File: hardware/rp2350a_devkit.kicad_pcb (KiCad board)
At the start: 2 copper layers, 29 x 60.5 mm, 55 parts, among them J1 USB_C_Receptacle_USB2.0_16P, J2 Conn_01x03, J3 Conn_01x16, J4 Conn_01x16, SW1 SW_Push, SW2 SW_Push, U1 NCP1117-3.3_SOT223, U2 USBLC6-2SC6, U3 W25Q128JVS, Y1 Crystal_GND24

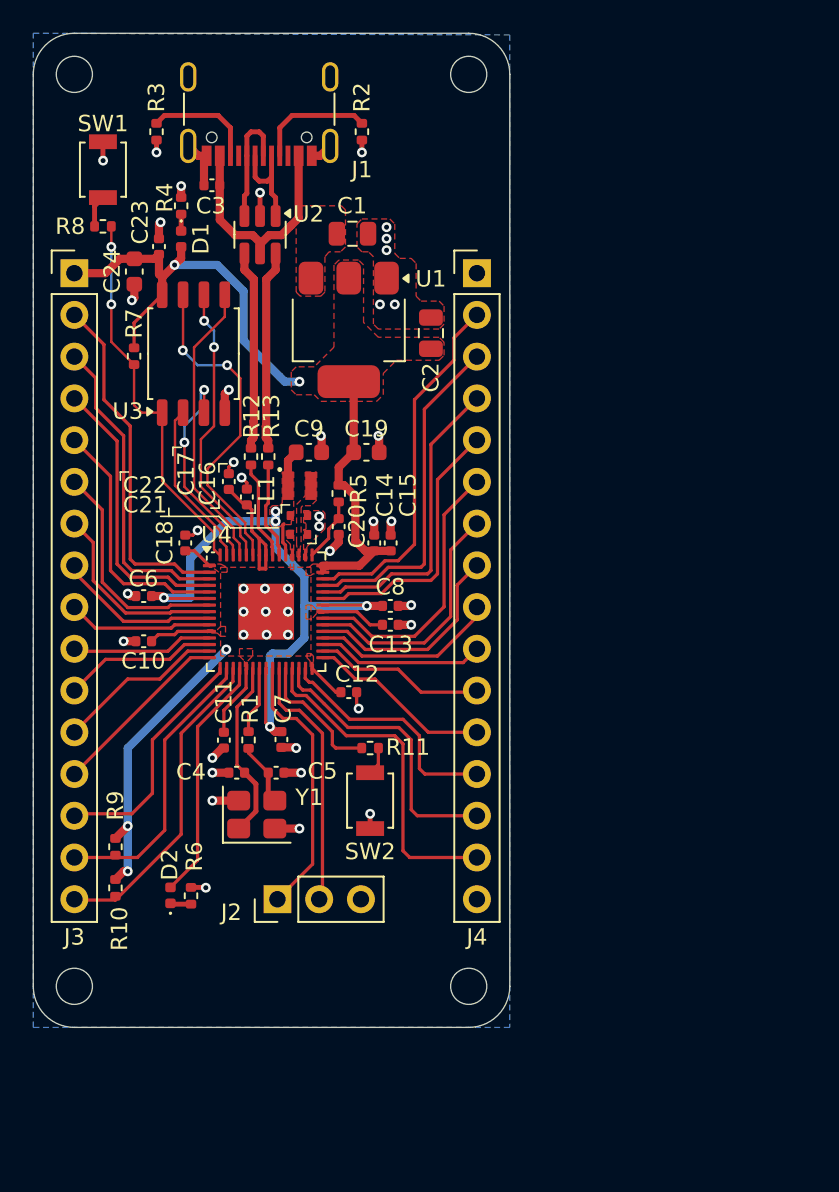
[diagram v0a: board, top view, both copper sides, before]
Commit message: add images and files for v1.0a
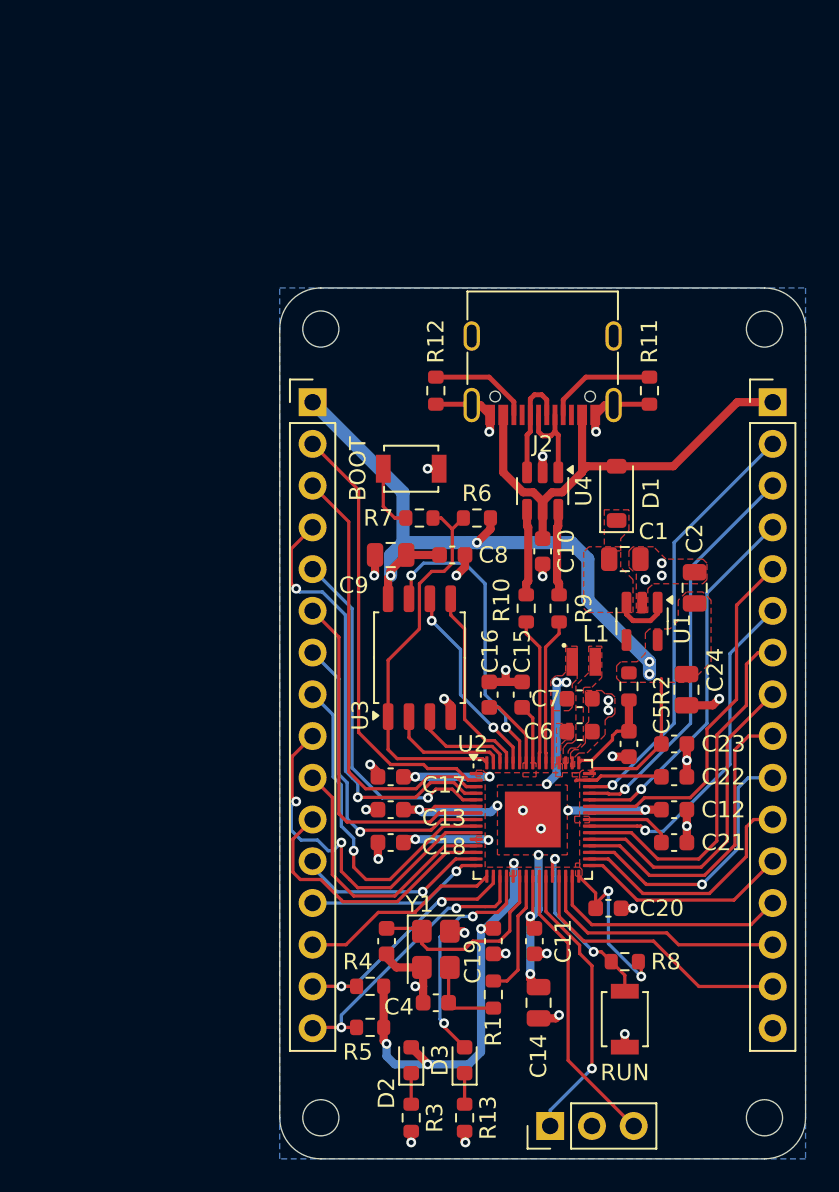
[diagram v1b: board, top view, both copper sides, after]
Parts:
- removed SW1, SW2: SW_Push, Button_Switch_SMD:SW_SPST_B3U-1000P
- added BOOT: SW_Push, Button_Switch_SMD:SW_SPST_B3U-1000P, F.Cu at (157.0, 107.0)
- added D3: LED, LED_SMD:LED_0603_1608Metric, F.Cu at (160.2, 143.0)
- added RUN: SW_Push, Button_Switch_SMD:SW_SPST_B3U-1000P, F.Cu at (170.0, 140.5)
- C10, C11, C12, C13, C15, C16, C17, C18, C23, C4, C8: footprint Capacitor_SMD:C_0402_1005Metric -> Capacitor_SMD:C_0603_1608Metric
- C14: value 100n -> 10u; footprint Capacitor_SMD:C_0402_1005Metric -> Capacitor_SMD:C_0805_2012Metric
- C19: value 10u -> 100n
- C20: value 4.7u -> 100n; footprint Capacitor_SMD:C_0402_1005Metric -> Capacitor_SMD:C_0603_1608Metric
- C21, C22: value 4.7u -> 100n; footprint footprints:C_0402_smallpads -> Capacitor_SMD:C_0603_1608Metric
- C24, C9: footprint Capacitor_SMD:C_0603_1608Metric -> Capacitor_SMD:C_0805_2012Metric
- C3: value 100n -> 15p; footprint Capacitor_SMD:C_0402_1005Metric -> Capacitor_SMD:C_0603_1608Metric
- C5: value 15p -> 4.7u; footprint Capacitor_SMD:C_0402_1005Metric -> Capacitor_SMD:C_0603_1608Metric
- C6: value 100u -> 4.7u; footprint Capacitor_SMD:C_0402_1005Metric -> Capacitor_SMD:C_0603_1608Metric
- C7: value 100n -> 4.7u; footprint Capacitor_SMD:C_0402_1005Metric -> Capacitor_SMD:C_0603_1608Metric
- D1: value LED -> D_Schottky; footprint LED_SMD:LED_0402_1005Metric -> Diode_SMD:D_SOD-123
- D2: footprint LED_SMD:LED_0402_1005Metric -> LED_SMD:LED_0603_1608Metric
- J1: value USB_C_Receptacle_USB2.0_16P -> Conn_01x03; footprint Connector_USB:USB_C_Receptacle_G-Switch_GT-USB-7010ASV -> Connector_PinHeader_2.54mm:PinHeader_1x03_P2.54mm_Vertical
- J2: value Conn_01x03 -> USB_C_Receptacle_USB2.0_16P; footprint Connector_PinHeader_2.54mm:PinHeader_1x03_P2.54mm_Vertical -> Connector_USB:USB_C_Receptacle_G-Switch_GT-USB-7010ASV
- R1: footprint Resistor_SMD:R_0402_1005Metric -> Resistor_SMD:R_0603_1608Metric
- R10, R9: value 10k -> 27; footprint Resistor_SMD:R_0402_1005Metric -> Resistor_SMD:R_0603_1608Metric
- R11: value 1k -> 5k1; footprint Resistor_SMD:R_0402_1005Metric -> Resistor_SMD:R_0603_1608Metric
- R12: value 27 -> 5k1; footprint Resistor_SMD:R_0402_1005Metric -> Resistor_SMD:R_0603_1608Metric
- R13: value 27 -> 1k; footprint Resistor_SMD:R_0402_1005Metric -> Resistor_SMD:R_0603_1608Metric
- R2: value 5k1 -> 33; footprint Resistor_SMD:R_0402_1005Metric -> Resistor_SMD:R_0603_1608Metric
- R3: value 5k1 -> 1k; footprint Resistor_SMD:R_0402_1005Metric -> Resistor_SMD:R_0603_1608Metric
- R4, R6, R8: value 1k -> 10k; footprint Resistor_SMD:R_0402_1005Metric -> Resistor_SMD:R_0603_1608Metric
- R5: value 33 -> 10k; footprint Resistor_SMD:R_0402_1005Metric -> Resistor_SMD:R_0603_1608Metric
- R7: value 10k -> 1k; footprint Resistor_SMD:R_0402_1005Metric -> Resistor_SMD:R_0603_1608Metric
- U1: value NCP1117-3.3_SOT223 -> AP2112K-3.3; footprint Package_TO_SOT_SMD:SOT-223-3_TabPin2 -> Package_TO_SOT_SMD:SOT-23-5
- U2: value USBLC6-2SC6 -> RP2350A; footprint Package_TO_SOT_SMD:SOT-23-6 -> Package_DFN_QFN:QFN-60-1EP_7x7mm_P0.4mm_EP3.4x3.4mm
- U4: value ~ -> USBLC6-2SC6; footprint Package_DFN_QFN:QFN-60-1EP_7x7mm_P0.4mm_EP3.4x3.4mm -> Package_TO_SOT_SMD:SOT-23-6
- moved H2 76.1 mm to (178.5, 146.5)
- moved J1 65.2 mm to (165.5, 147.0), turned to 90 degrees
- moved R3 62.0 mm to (157.0, 146.5)
- moved R8 54.9 mm to (170.0, 137.0)
- moved R4 48.9 mm to (154.5, 138.5), turned to 0 degrees
- moved C3 47.2 mm to (155.5, 135.8), turned to -90 degrees
- moved C23 43.6 mm to (173.0, 123.8), turned to 0 degrees
- moved C24 42.2 mm to (173.8, 120.5)
- moved R13 42.0 mm to (160.2, 146.5), turned to -90 degrees
- moved H4 41.0 mm to (151.5, 98.5)
- moved U2 39.3 mm to (164.4, 128.3), turned to 0 degrees
- moved R2 37.5 mm to (170.2, 120.2)
- moved J2 36.9 mm to (165.0, 100.0), turned to 180 degrees
- moved R5 32.5 mm to (154.5, 141.0), turned to 0 degrees
- moved C19 30.7 mm to (162.0, 135.8), turned to -90 degrees
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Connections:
- C1 pad 1: VBUS -> /5VIN
- C10 pad 1: +3V3 -> VBUS
- C11 pad 1: +3V3 -> +1V1
- C12 pad 1: +3V3 -> +1V1
- C13 pad 1: +3V3 -> +1V1
- C14 pad 1: +3V3 -> +1V1
- C20 pad 1: /VREG_AVDD -> +3V3
- C22 pad 1: +1V1 -> +3V3
- C3 pad 1: VBUS -> /XIN
- C4 pad 1: /XIN -> /XTAL_OUT
- C5 pad 1: /XTAL_OUT -> /VREG_AVDD
- C6 pad 1: +1V1 -> +3V3
- C8 pad 1: +1V1 -> +3V3
- C9 pad 1: +1V1 -> +3V3
- D1 pad 1: Net-(D1-K) -> /5VIN
- D1 pad 2: +3V3 -> VBUS
- D2 pad 1: Net-(D2-K) -> /POWER_LED
- D2 pad 2: /IO15 -> +3V3
- J4 pad 1: GND -> VBUS
- J4 pad 16: unconnected-(J4-Pin_16-Pad16) -> GND
- R10 pad 1: /IO14/SDA -> /USB_R+
- R10 pad 2: +3V3 -> /USB_DOUT+
- R11 pad 1: /RUN_SW -> /CC1
- R11 pad 2: Net-(U4-RUN) -> GND
- R12 pad 1: /USB_R+ -> /CC2
- R12 pad 2: /USB_DOUT+ -> GND
- R13 pad 1: /USB_R- -> Net-(D3-K)
- R13 pad 2: /USB_DOUT- -> GND
- R2 pad 1: /CC1 -> +3V3
- R2 pad 2: GND -> /VREG_AVDD
- R3 pad 1: /CC2 -> /POWER_LED
- R4 pad 1: Net-(D1-K) -> /IO13/SCL
- R4 pad 2: GND -> +3V3
- R5 pad 1: +3V3 -> /IO14/SDA
- R5 pad 2: /VREG_AVDD -> +3V3
- R6 pad 1: Net-(D2-K) -> +3V3
- R6 pad 2: GND -> /QSPI_SS
- R7 pad 1: +3V3 -> /BOOT_SW
- R8 pad 1: /BOOT_SW -> /RUN_SW
- R8 pad 2: /QSPI_SS -> +3V3
- R9 pad 1: /IO13/SCL -> /USB_R-
- R9 pad 2: +3V3 -> /USB_DOUT-
- U1 pad 1: GND -> /5VIN
- U1 pad 2: +3V3 -> GND
- U1 pad 3: VBUS -> /5VIN
- U2 pad 1: /USB_DIN- -> +3V3
- U2 pad 2: GND -> /IO00
- U2 pad 3: /USB_DIN+ -> /IO01
- U2 pad 4: /USB_DOUT+ -> /IO02
- U2 pad 5: VBUS -> /IO03
- U2 pad 6: /USB_DOUT- -> +1V1
- U4 pad 1: +3V3 -> /USB_DIN-
- U4 pad 2: /IO00 -> GND
- U4 pad 3: /IO01 -> /USB_DIN+
- U4 pad 4: /IO02 -> /USB_DOUT+
- U4 pad 5: /IO03 -> VBUS
- U4 pad 6: +1V1 -> /USB_DOUT-
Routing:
- net +3V3: track 87.4 -> 115.3 mm, vias 5 -> 14
- net VBUS: track 14.9 -> 28.9 mm
- net /IO07: track 8.83 -> 22.0 mm, vias 0 -> 2
- net /IO06: track 9.96 -> 20.7 mm, vias 0 -> 1
- net /IO02: track 17.3 -> 27.3 mm, vias 0 -> 2
- net /RUN_SW: track 1.71 -> 11.2 mm, vias 0 -> 2
- net /IO08: track 8.61 -> 16.9 mm
- net Net-(U4-RUN): track 8.18 -> 0.00 mm
- net /IO04: track 14.0 -> 21.8 mm
- net /IO01: track 19.4 -> 27.1 mm
- net /IO05: track 11.9 -> 19.5 mm, vias 0 -> 1
- net /IO22: track 11.4 -> 18.9 mm
- net /IO09: track 9.37 -> 16.8 mm
- net /IO24: track 15.3 -> 22.3 mm
- net /QSPI_SD2: track 13.2 -> 6.21 mm, vias 2 -> 0
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- added copper zone on F.Cu, net /5VIN
- removed copper zone on F.Cu, net VBUS
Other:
- board size 29 x 60.5 mm -> 32 x 53 mm
- board text added: "3V3"
- board text added: "5V"
- board text added: "IOA0"
- board text added: "IOA1"
- board text added: "IOA2"
- board text added: "IOA3"
- board text added: "SWCLK"
- board text added: "SWDIO"
- board text removed: "+3V3"
- board text removed: "A0"
- board text removed: "A1"
- board text removed: "A2"
- board text removed: "A3"
- board text removed: "NC"
